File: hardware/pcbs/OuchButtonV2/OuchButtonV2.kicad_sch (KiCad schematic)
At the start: 77 parts, among them J1 USB_C_Receptacle_USB2.0_14P, J3 Conn_01x01_Pin, Q1 AO3423 P-Chanel, U1 ESP32-C6-MINI-1/U, U2 RT9080-33GJ5, U3 MCP73831-2-OT, U4 MPU-6050, U5 DS1307Z+, U6 AT42QT1010-TSHR, U7 TS3A24159DGS, U8 AFE4404YZPT, U9 WE-TVS-82400102, Y1 32.768 kHz

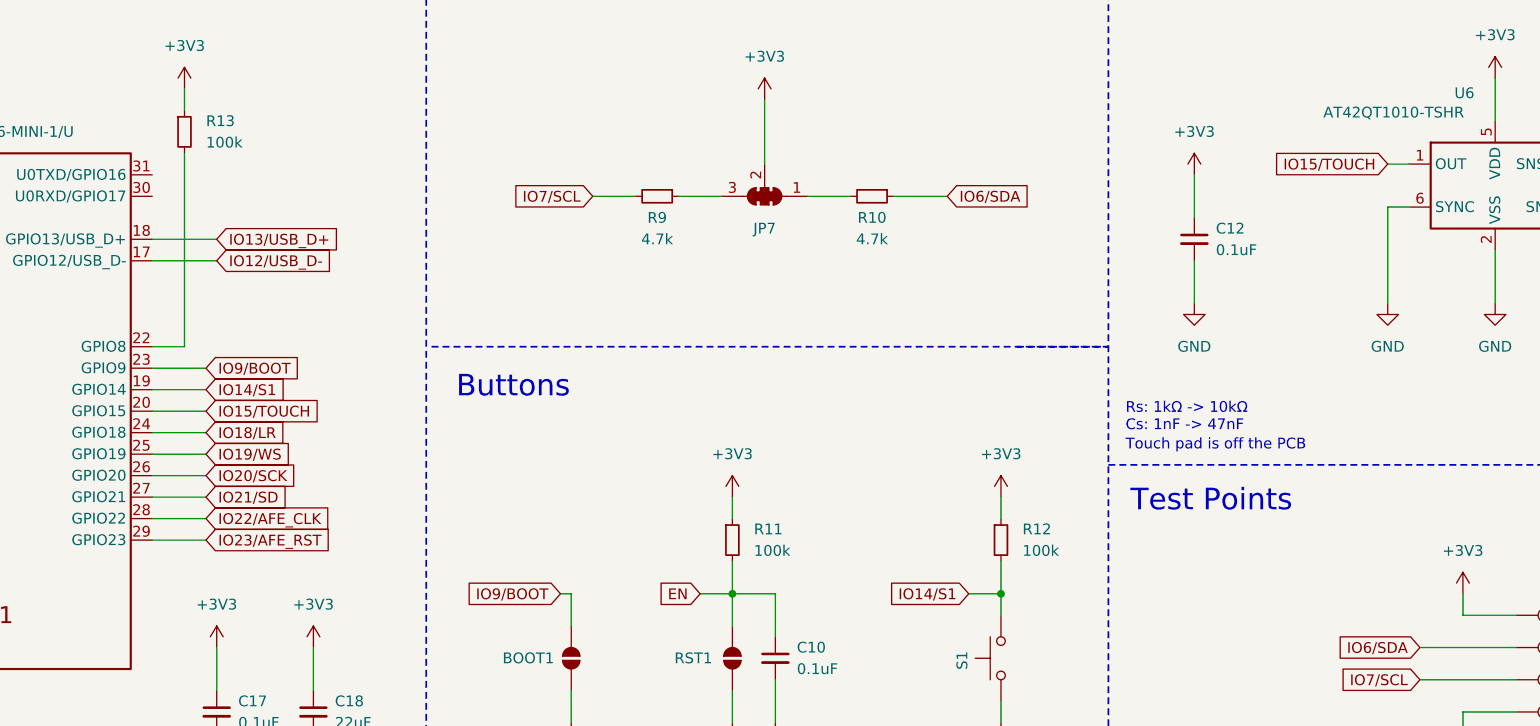
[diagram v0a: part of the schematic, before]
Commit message: Half done pcb
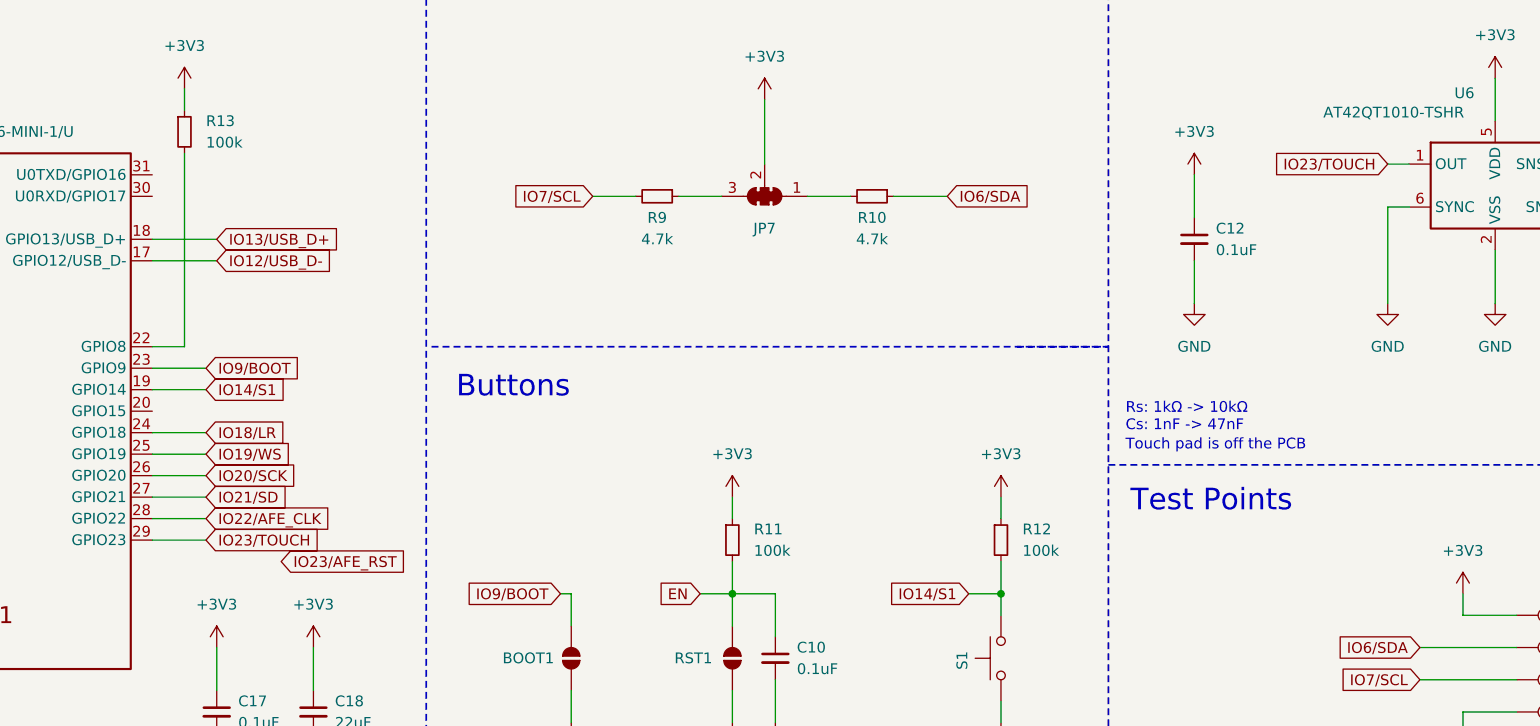
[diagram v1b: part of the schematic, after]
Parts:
- C1, C10, C11, C12, C13, C14, C15, C16, C17, C18, C2, C3, C4, C5, C6, C7, C8, C9: footprint Capacitor_SMD:C_0603_1608Metric_Pad1.08x0.95mm_HandSolder -> Capacitor_SMD:C_0805_2012Metric
- D1: footprint Diode_SMD:D_0603_1608Metric_Pad1.05x0.95mm_HandSolder -> Diode_SMD:D_0805_2012Metric
- D2: footprint LED_SMD:LED_0603_1608Metric_Pad1.05x0.95mm_HandSolder -> LED_SMD:LED_0805_2012Metric
- R1, R10, R11, R12, R13, R14, R15, R16, R17, R18, R2, R3, R4, R5, R6, R7, R9: footprint Resistor_SMD:R_0603_1608Metric_Pad0.98x0.95mm_HandSolder -> Resistor_SMD:R_0805_2012Metric
- R19, R20, R8: footprint Resistor_SMD:R_0603_1608Metric_Pad0.98x0.95mm_HandSolder -> Capacitor_SMD:C_0805_2012Metric
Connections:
- net IO23/AFE_RST: no longer U1.29 (GPIO23)
- net IO15/TOUCH: no longer names the net of U1.20 (GPIO15)
- net IO15/TOUCH: no longer U6.1 (OUT)
- new net IO23/TOUCH: U1.29 (GPIO23), U6.1 (OUT)
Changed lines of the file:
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@@
 	(wire
 		(pts
-			(xy 91.44 232.41) (xy 97.79 232.41)
-		)
-		(stroke
-			(width 0)
-			(type default)
-		)
-	)
-	(wire
-		(pts
 			(xy 187.96 254) (xy 191.77 254)
 		)
@@
 	(wire
 		(pts
+			(xy 91.44 247.65) (xy 97.79 247.65)
+		)
+		(stroke
+			(width 0)
+			(type default)
+		)
+	)
+	(wire
+		(pts
 			(xy 241.3 264.16) (xy 252.73 264.16)
 		)
@@
 	(wire
 		(pts
-			(xy 91.44 247.65) (xy 97.79 247.65)
-		)
-		(stroke
-			(width 0)
-			(type default)
-		)
-	)
-	(wire
-		(pts
 			(xy 201.93 63.5) (xy 201.93 69.85)
 		)
@@
 		)
 	)
-	(global_label "IO15{slash}TOUCH"
+	(global_label "IO23{slash}TOUCH"
 		(shape input)
-		(at 97.79 232.41 0)
+		(at 97.79 247.65 0)
 		(fields_autoplaced yes)
 		(effects
@@
 		)
 		(property "Intersheetrefs" "${INTERSHEET_REFS}"
-			(at 112.6891 232.41 0)
+			(at 112.6891 247.65 0)
 			(effects
 				(font
@@
 		)
 	)
-	(global_label "IO15{slash}TOUCH"
+	(global_label "IO23{slash}TOUCH"
 		(shape input)
 		(at 237.49 203.2 180)
@@
 	(global_label "IO23{slash}AFE_RST"
 		(shape input)
-		(at 97.79 247.65 0)
+		(at 106.68 250.19 0)
 		(fields_autoplaced yes)
 		(effects
@@
 		)
 		(property "Intersheetrefs" "${INTERSHEET_REFS}"
-			(at 114.2009 247.65 0)
+			(at 123.0909 250.19 0)
 			(effects
 				(font
@@
 			)
 		)
-		(property "Footprint" "Resistor_SMD:R_0603_1608Metric_Pad0.98x0.95mm_HandSolder"
+		(property "Footprint" "Resistor_SMD:R_0805_2012Metric"
 			(at 151.13 207.01 0)
 			(effects
@@
 			)
 		)
-		(property "Footprint" "Resistor_SMD:R_0603_1608Metric_Pad0.98x0.95mm_HandSolder"
+		(property "Footprint" "Resistor_SMD:R_0805_2012Metric"
 			(at 160.02 247.65 0)
 			(effects
@@
 			)
 		)
-		(property "Footprint" "Resistor_SMD:R_0603_1608Metric_Pad0.98x0.95mm_HandSolder"
+		(property "Footprint" "Resistor_SMD:R_0805_2012Metric"
 			(at 383.54 128.27 0)
 			(effects
@@
 			)
 		)
-		(property "Footprint" "Capacitor_SMD:C_0603_1608Metric_Pad1.08x0.95mm_HandSolder"
+		(property "Footprint" "Capacitor_SMD:C_0805_2012Metric"
 			(at 236.22 161.29 0)
 			(effects
@@
 			)
 		)
-		(property "Footprint" "Capacitor_SMD:C_0603_1608Metric_Pad1.08x0.95mm_HandSolder"
+		(property "Footprint" "Capacitor_SMD:C_0805_2012Metric"
 			(at 165.1 261.62 0)
 			(effects
@@
 			)
 		)
-		(property "Footprint" "Resistor_SMD:R_0603_1608Metric_Pad0.98x0.95mm_HandSolder"
+		(property "Footprint" "Resistor_SMD:R_0805_2012Metric"
 			(at 176.53 207.01 0)
 			(effects
@@
 			)
 		)
-		(property "Footprint" "Resistor_SMD:R_0603_1608Metric_Pad0.98x0.95mm_HandSolder"
+		(property "Footprint" "Resistor_SMD:R_0805_2012Metric"
 			(at 207.01 165.1 0)
 			(effects
@@
 			)
 		)
-		(property "Footprint" "Resistor_SMD:R_0603_1608Metric_Pad0.98x0.95mm_HandSolder"
+		(property "Footprint" "Resistor_SMD:R_0805_2012Metric"
 			(at 213.36 63.5 0)
 			(effects
@@
 			)
 		)
-		(property "Footprint" "Resistor_SMD:R_0603_1608Metric_Pad0.98x0.95mm_HandSolder"
+		(property "Footprint" "Resistor_SMD:R_0805_2012Metric"
 			(at 95.25 199.39 0)
 			(effects
@@
 			)
 		)
-		(property "Footprint" "Capacitor_SMD:C_0603_1608Metric_Pad1.08x0.95mm_HandSolder"
+		(property "Footprint" "Capacitor_SMD:C_0805_2012Metric"
 			(at 274.32 60.96 0)
 			(effects
@@
 			)
 		)
-		(property "Footprint" "LED_SMD:LED_0603_1608Metric_Pad1.05x0.95mm_HandSolder"
+		(property "Footprint" "LED_SMD:LED_0805_2012Metric"
 			(at 370.84 231.14 0)
 			(effects
@@
 			)
 		)
-		(property "Footprint" "Capacitor_SMD:C_0603_1608Metric_Pad1.08x0.95mm_HandSolder"
+		(property "Footprint" "Capacitor_SMD:C_0805_2012Metric"
 			(at 105.41 143.51 0)
 			(effects
@@
 			)
 		)
-		(property "Footprint" "Capacitor_SMD:C_0603_1608Metric_Pad1.08x0.95mm_HandSolder"
+		(property "Footprint" "Capacitor_SMD:C_0805_2012Metric"
 			(at 267.97 204.47 0)
 			(effects
@@
 			)
 		)
-		(property "Footprint" "Resistor_SMD:R_0603_1608Metric_Pad0.98x0.95mm_HandSolder"
+		(property "Footprint" "Capacitor_SMD:C_0805_2012Metric"
 			(at 58.42 40.64 0)
 			(effects
@@
 			)
 		)
-		(property "Footprint" "Resistor_SMD:R_0603_1608Metric_Pad0.98x0.95mm_HandSolder"
+		(property "Footprint" "Resistor_SMD:R_0805_2012Metric"
 			(at 280.67 199.39 0)
 			(effects
@@
 			)
 		)
-		(property "Footprint" "Capacitor_SMD:C_0603_1608Metric_Pad1.08x0.95mm_HandSolder"
+		(property "Footprint" "Capacitor_SMD:C_0805_2012Metric"
 			(at 173.99 43.18 0)
 			(effects
@@
 			)
 		)
-		(property "Footprint" "Capacitor_SMD:C_0603_1608Metric_Pad1.08x0.95mm_HandSolder"
+		(property "Footprint" "Capacitor_SMD:C_0805_2012Metric"
 			(at 110.49 267.97 0)
 			(effects
@@
 			)
 		)
-		(property "Footprint" "Resistor_SMD:R_0603_1608Metric_Pad0.98x0.95mm_HandSolder"
+		(property "Footprint" "Resistor_SMD:R_0805_2012Metric"
 			(at 285.75 40.64 0)
 			(effects
@@
 			)
 		)
-		(property "Footprint" "Resistor_SMD:R_0603_1608Metric_Pad0.98x0.95mm_HandSolder"
+		(property "Footprint" "Resistor_SMD:R_0805_2012Metric"
 			(at 191.77 247.65 0)
 			(effects
@@
 			)
 		)
-		(property "Footprint" "Capacitor_SMD:C_0603_1608Metric_Pad1.08x0.95mm_HandSolder"
+		(property "Footprint" "Capacitor_SMD:C_0805_2012Metric"
 			(at 383.54 173.99 0)
 			(effects
@@
 			)
 		)
-		(property "Footprint" "Capacitor_SMD:C_0603_1608Metric_Pad1.08x0.95mm_HandSolder"
+		(property "Footprint" "Capacitor_SMD:C_0805_2012Metric"
 			(at 152.4 52.07 0)
 			(effects
@@
 			)
 		)
-		(property "Footprint" "Resistor_SMD:R_0603_1608Metric_Pad0.98x0.95mm_HandSolder"
+		(property "Footprint" "Resistor_SMD:R_0805_2012Metric"
 			(at 373.38 135.89 0)
 			(effects
@@
 			)
 		)
-		(property "Footprint" "Capacitor_SMD:C_0603_1608Metric_Pad1.08x0.95mm_HandSolder"
+		(property "Footprint" "Capacitor_SMD:C_0805_2012Metric"
 			(at 116.84 143.51 0)
 			(effects
@@
 			)
 		)
-		(property "Footprint" "Resistor_SMD:R_0603_1608Metric_Pad0.98x0.95mm_HandSolder"
+		(property "Footprint" "Capacitor_SMD:C_0805_2012Metric"
 			(at 58.42 38.1 0)
 			(effects
@@
 			)
 		)
-		(property "Footprint" "Resistor_SMD:R_0603_1608Metric_Pad0.98x0.95mm_HandSolder"
+		(property "Footprint" "Resistor_SMD:R_0805_2012Metric"
 			(at 45.72 59.69 0)
 			(effects
@@
 			)
 		)
-		(property "Footprint" "Capacitor_SMD:C_0603_1608Metric_Pad1.08x0.95mm_HandSolder"
+		(property "Footprint" "Capacitor_SMD:C_0805_2012Metric"
 			(at 394.97 173.99 0)
 			(effects
@@
 			)
 		)
-		(property "Footprint" "Capacitor_SMD:C_0603_1608Metric_Pad1.08x0.95mm_HandSolder"
+		(property "Footprint" "Capacitor_SMD:C_0805_2012Metric"
 			(at 113.03 53.34 0)
 			(effects
@@
 			)
 		)
-		(property "Footprint" "Resistor_SMD:R_0603_1608Metric_Pad0.98x0.95mm_HandSolder"
+		(property "Footprint" "Resistor_SMD:R_0805_2012Metric"
 			(at 186.69 53.34 0)
 			(effects
@@
 			)
 		)
-		(property "Footprint" "Resistor_SMD:R_0603_1608Metric_Pad0.98x0.95mm_HandSolder"
+		(property "Footprint" "Resistor_SMD:R_0805_2012Metric"
 			(at 383.54 142.24 0)
 			(effects
@@
 			)
 		)
-		(property "Footprint" "Diode_SMD:D_0603_1608Metric_Pad1.05x0.95mm_HandSolder"
+		(property "Footprint" "Diode_SMD:D_0805_2012Metric"
 			(at 96.52 45.72 0)
 			(effects
@@
 			)
 		)
-		(property "Footprint" "Capacitor_SMD:C_0603_1608Metric_Pad1.08x0.95mm_HandSolder"
+		(property "Footprint" "Capacitor_SMD:C_0805_2012Metric"
 			(at 370.84 173.99 0)
 			(effects
@@
 			)
 		)
-		(property "Footprint" "Resistor_SMD:R_0603_1608Metric_Pad0.98x0.95mm_HandSolder"
+		(property "Footprint" "Capacitor_SMD:C_0805_2012Metric"
 			(at 102.87 53.34 0)
 			(effects
@@
 			)
 		)
-		(property "Footprint" "Resistor_SMD:R_0603_1608Metric_Pad0.98x0.95mm_HandSolder"
+		(property "Footprint" "Resistor_SMD:R_0805_2012Metric"
 			(at 125.73 49.53 0)
 			(effects
@@
 			)
 		)
-		(property "Footprint" "Resistor_SMD:R_0603_1608Metric_Pad0.98x0.95mm_HandSolder"
+		(property "Footprint" "Resistor_SMD:R_0805_2012Metric"
 			(at 285.75 60.96 0)
 			(effects
@@
 			)
 		)
-		(property "Footprint" "Capacitor_SMD:C_0603_1608Metric_Pad1.08x0.95mm_HandSolder"
+		(property "Footprint" "Capacitor_SMD:C_0805_2012Metric"
 			(at 223.52 63.5 0)
 			(effects
@@
 			)
 		)
-		(property "Footprint" "Resistor_SMD:R_0603_1608Metric_Pad0.98x0.95mm_HandSolder"
+		(property "Footprint" "Resistor_SMD:R_0805_2012Metric"
 			(at 54.61 59.69 0)
 			(effects
@@
 			)
 		)
-		(property "Footprint" "Capacitor_SMD:C_0603_1608Metric_Pad1.08x0.95mm_HandSolder"
+		(property "Footprint" "Capacitor_SMD:C_0805_2012Metric"
 			(at 214.63 212.09 0)
 			(effects
@@
 			)
 		)
-		(property "Footprint" "Capacitor_SMD:C_0603_1608Metric_Pad1.08x0.95mm_HandSolder"
+		(property "Footprint" "Capacitor_SMD:C_0805_2012Metric"
 			(at 127 143.51 0)
 			(effects
@@
 			)
 		)
-		(property "Footprint" "Capacitor_SMD:C_0603_1608Metric_Pad1.08x0.95mm_HandSolder"
+		(property "Footprint" "Capacitor_SMD:C_0805_2012Metric"
 			(at 93.98 143.51 0)
 			(effects
@@
 			)
 		)
-		(property "Footprint" "Capacitor_SMD:C_0603_1608Metric_Pad1.08x0.95mm_HandSolder"
+		(property "Footprint" "Capacitor_SMD:C_0805_2012Metric"
 			(at 99.06 267.97 0)
 			(effects

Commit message: Ready for review pcb
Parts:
- removed JP1, JP2: SolderJumper_2_Bridged, Jumper:SolderJumper-2_P1.3mm_Open_RoundedPad1.0x1.5mm, symbol Jumper:SolderJumper_2_Bridged
- removed JP7: SolderJumper_3_Bridged123, Jumper:SolderJumper-3_P1.3mm_Open_RoundedPad1.0x1.5mm_NumberLabels, symbol Jumper:SolderJumper_3_Bridged123
- U7: footprint Package_CSP:LFCSP-16-1EP_4x4mm_P0.65mm_EP2.1x2.1mm -> Package_SO:TSSOP-10_3x3mm_P0.5mm
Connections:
- net IO23/AFE_RST is gone; now on net IO15/AFE_RST: R17.2, U8.D1 (RESETZ)
- net +3V3: now also R10.1, R9.1
- net IO6/SDA: now also R10.2; no longer R10.1
- net at J1.A7 (D-): now also J1.B7 (D-), R19.2
- net at J1.A6 (D+), R20.2: now also J1.B6 (D+)
- net IO15/AFE_RST: now reaches U1.20 (GPIO15)
- net IO14/S1 renamed IO21/S1
- net IO21/S1: now also U1.27 (GPIO21); no longer U1.19 (GPIO14)
- net IO21/SD renamed IO14/SD
- net IO14/SD: now also U1.19 (GPIO14); no longer U1.27 (GPIO21)
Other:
- moved on the sheet: R10, R19, R20, R9

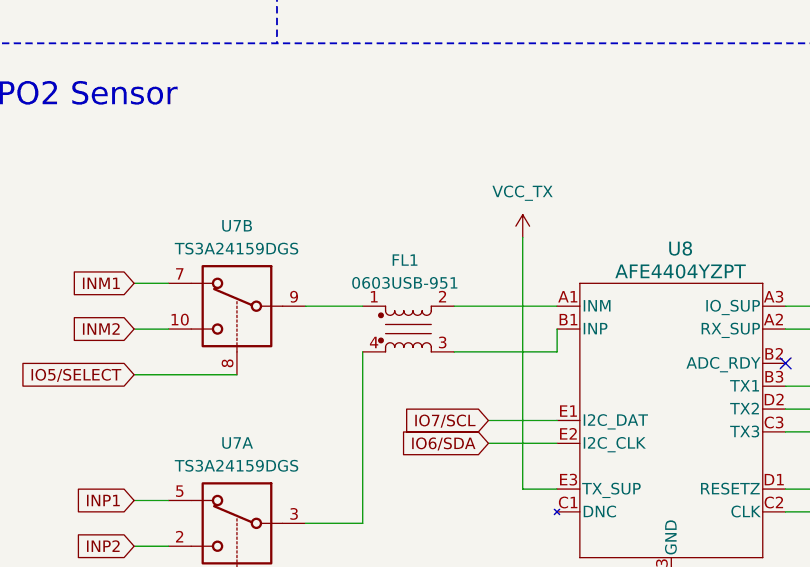
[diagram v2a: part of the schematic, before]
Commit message: For manufacturing
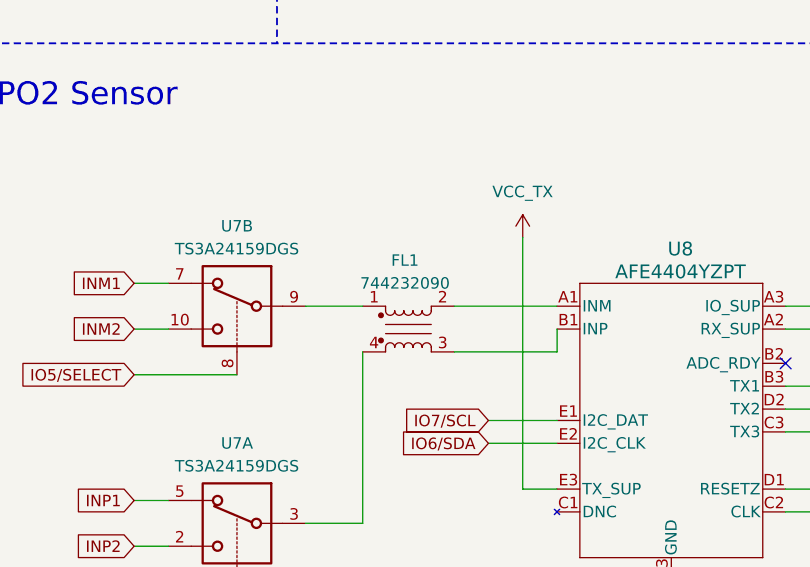
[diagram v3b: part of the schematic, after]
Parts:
- D1: footprint Diode_SMD:D_0805_2012Metric -> Diode_SMD:D_SOD-323
- FL1: value 0603USB-951 -> 744232090
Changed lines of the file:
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@@
 			)
 		)
-		(property "Value" "0603USB-951"
+		(property "Value" "744232090"
 			(at 324.739 110.49 0)
 			(effects
@@
 			)
 		)
-		(property "Datasheet" "https://www.coilcraft.com/pdfs/0603usb.pdf"
+		(property "Datasheet" "CMC 370MA 2LN 90OHM SMD AEC-Q200"
 			(at 325.12 123.825 0)
 			(effects
@@
 			)
 		)
-		(property "Footprint" "Diode_SMD:D_0805_2012Metric"
+		(property "Footprint" "Diode_SMD:D_SOD-323"
 			(at 96.52 45.72 0)
 			(effects
